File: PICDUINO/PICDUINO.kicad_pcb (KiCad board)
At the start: 2 copper layers, 42 parts, among them J1 Conn_01x03_Female, J10 Conn_01x03_Female, J2 Conn_01x14_Female, J3 Conn_01x05_Male, J4 Conn_01x02_Male, J5 Conn_01x04_Male, J6 Conn_01x16_Male, J7 Barrel_Jack_Switch, J8 Conn_01x03_Female, J9 Conn_01x03_Female, K1 FINDER-36.11, K2 FINDER-36.11, K3 FINDER-36.11, K4 FINDER-36.11, Q1 BC337, SW1 SW_Push, U1 L7805, U2 PIC18F4550-IP, U3 ULN2003, U4 HEF4094BP, Y1 Crystal

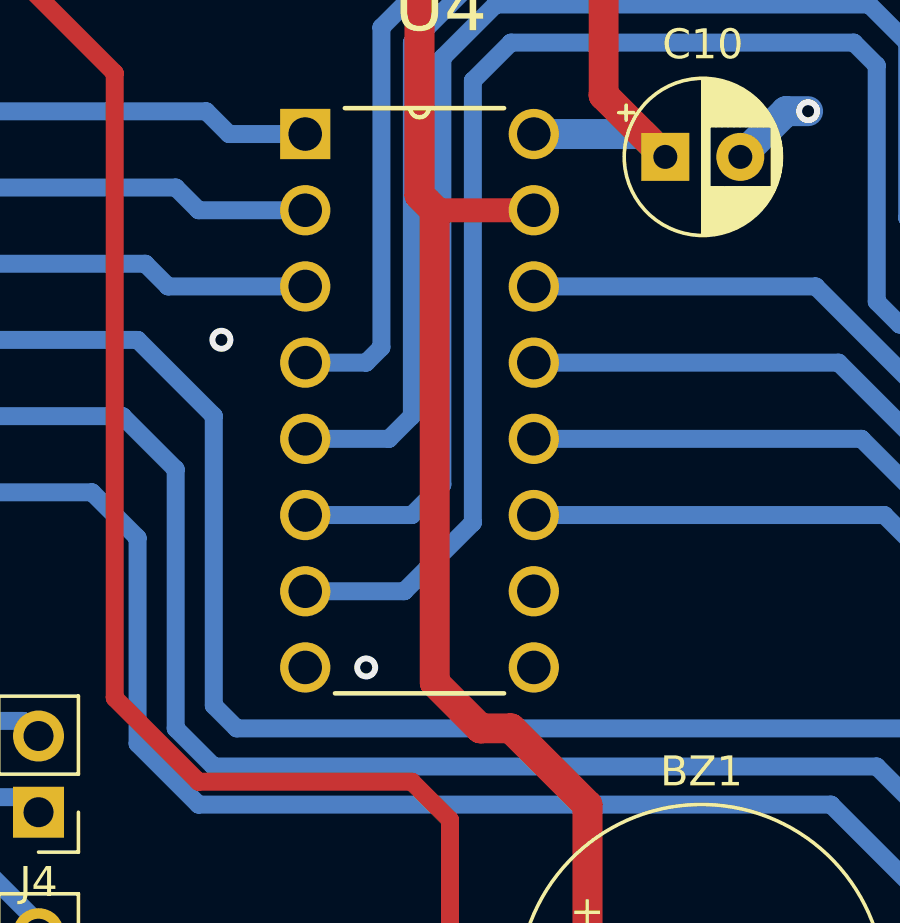
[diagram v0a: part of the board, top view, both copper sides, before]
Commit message: Add files via upload
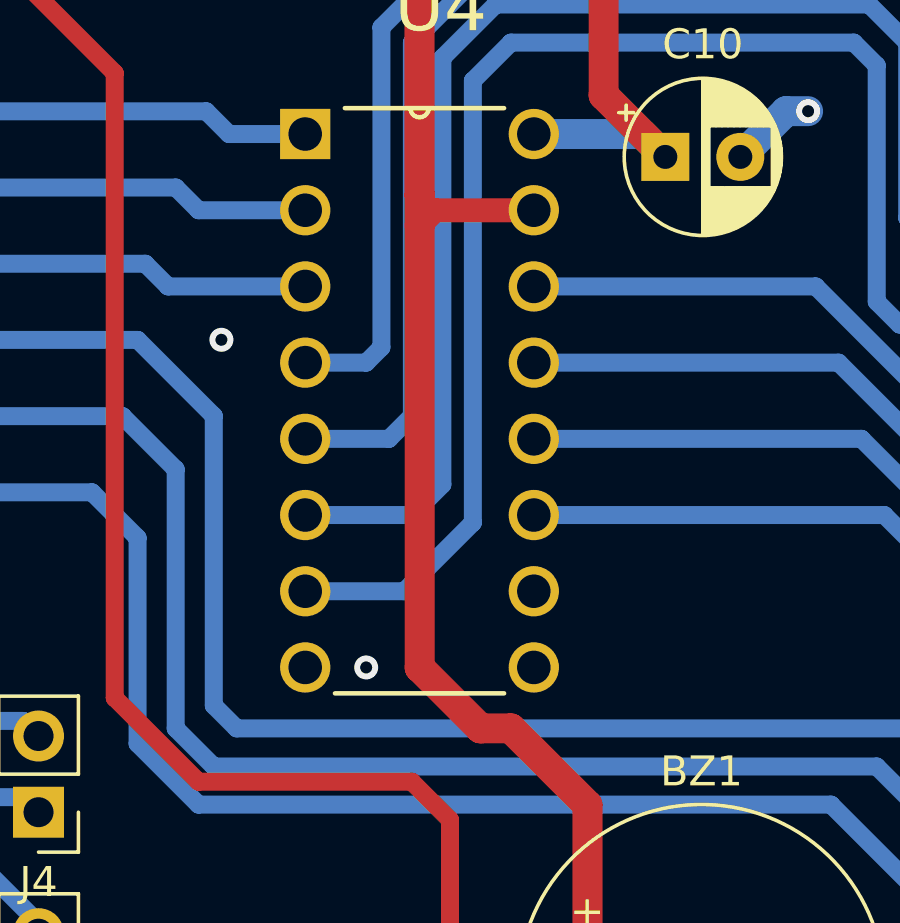
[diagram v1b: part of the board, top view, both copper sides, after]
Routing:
- net /VDD: track 300.2 -> 300.9 mm
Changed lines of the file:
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@@
   (segment (start 162.814 79.65) (end 164.698 79.65) (width 0.8) (layer "F.Cu") (net 1))
   (segment (start 166.37 70.114) (end 165.344 69.088) (width 0.8) (layer "F.Cu") (net 1))
+  (segment (start 155.194 60.452) (end 157.744 63.002) (width 1) (layer "F.Cu") (net 2))
   (segment (start 135.636 107.95) (end 138.684 104.902) (width 1) (layer "F.Cu") (net 2))
-  (segment (start 152.4 42.926) (end 152.654 43.18) (width 1) (layer "F.Cu") (net 2))
   (segment (start 138.43 29.21) (end 138.43 30.988) (width 0.8) (layer "F.Cu") (net 2))
   (segment (start 155.956 74.422) (end 157.744 72.634) (width 1) (layer "F.Cu") (net 2))
-  (segment (start 154.178 60.452) (end 155.194 60.452) (width 1) (layer "F.Cu") (net 2))
-  (segment (start 157.744 63.002) (end 157.744 69.088) (width 1) (layer "F.Cu") (net 2))
-  (segment (start 155.956 43.18) (end 152.654 43.18) (width 0.8) (layer "F.Cu") (net 2))
+  (segment (start 152.15 43.684) (end 152.15 42.676) (width 1) (layer "F.Cu") (net 2))
   (segment (start 146.558 74.422) (end 155.956 74.422) (width 1) (layer "F.Cu") (net 2))
   (segment (start 142.24 34.798) (end 151.384 34.798) (width 0.8) (layer "F.Cu") (net 2))
   (segment (start 138.43 30.988) (end 142.24 34.798) (width 0.8) (layer "F.Cu") (net 2))
+  (segment (start 154.178 60.452) (end 155.194 60.452) (width 1) (layer "F.Cu") (net 2))
   (segment (start 153.67 32.512) (end 153.67 26.67) (width 1) (layer "F.Cu") (net 2))
+  (segment (start 152.146 42.672) (end 152.146 35.56) (width 1) (layer "F.Cu") (net 2))
   (segment (start 157.744 72.634) (end 157.744 69.088) (width 1) (layer "F.Cu") (net 2))
   (segment (start 138.684 82.296) (end 146.558 74.422) (width 1) (layer "F.Cu") (net 2))
+  (segment (start 152.15 43.684) (end 152.15 58.424) (width 1) (layer "F.Cu") (net 2))
+  (segment (start 152.654 43.18) (end 152.15 43.684) (width 0.8) (layer "F.Cu") (net 2))
   (segment (start 152.146 35.56) (end 151.384 34.798) (width 1) (layer "F.Cu") (net 2))
-  (segment (start 152.654 58.928) (end 154.178 60.452) (width 1) (layer "F.Cu") (net 2))
+  (segment (start 157.744 63.002) (end 157.744 69.088) (width 1) (layer "F.Cu") (net 2))
+  (segment (start 152.15 42.676) (end 152.146 42.672) (width 1) (layer "F.Cu") (net 2))
+  (segment (start 152.15 58.424) (end 154.178 60.452) (width 1) (layer "F.Cu") (net 2))
+  (segment (start 155.956 43.18) (end 152.654 43.18) (width 0.8) (layer "F.Cu") (net 2))
   (segment (start 151.384 34.798) (end 153.67 32.512) (width 1) (layer "F.Cu") (net 2))
-  (segment (start 152.146 42.672) (end 152.146 35.56) (width 1) (layer "F.Cu") (net 2))
-  (segment (start 152.654 43.18) (end 152.654 58.928) (width 1) (layer "F.Cu") (net 2))
   (segment (start 128.27 107.95) (end 135.636 107.95) (width 1) (layer "F.Cu") (net 2))
-  (segment (start 155.194 60.452) (end 157.744 63.002) (width 1) (layer "F.Cu") (net 2))
-  (segment (start 152.4 42.926) (end 152.146 42.672) (width 1) (layer "F.Cu") (net 2))
   (segment (start 138.684 104.902) (end 138.684 82.296) (width 1) (layer "F.Cu") (net 2))
   (segment (start 128.27 128.016) (end 128.27 107.95) (width 1) (layer "B.Cu") (net 2))
@@
   (segment (start 106.68 140.177) (end 108.204 141.701) (width 1) (layer "B.Cu") (net 81))
   (zone (net 3) (net_name "/VSS") (layers "F&B.Cu") (hatch edge 0.508)
-    (connect_pads yes (clearance 0.508))
-    (min_thickness 0.254) (filled_areas_thickness no)
-    (fill yes (thermal_gap 0.508) (thermal_bridge_width 0.508))
+    (connect_pads yes (clearance 0.25))
+    (min_thickness 0.1) (filled_areas_thickness no)
+    (fill yes (thermal_gap 0.2) (thermal_bridge_width 0.2))
     (polygon
       (pts
